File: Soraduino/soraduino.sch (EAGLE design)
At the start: 21 parts, among them IC1 ATMEGA168-AU, IC2 317EMP, IC3 317EMP

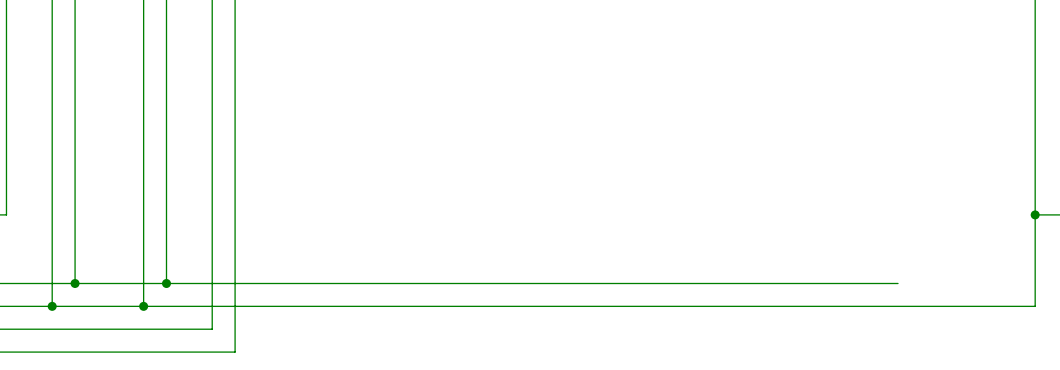
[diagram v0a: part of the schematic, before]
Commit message: 仮配線完了
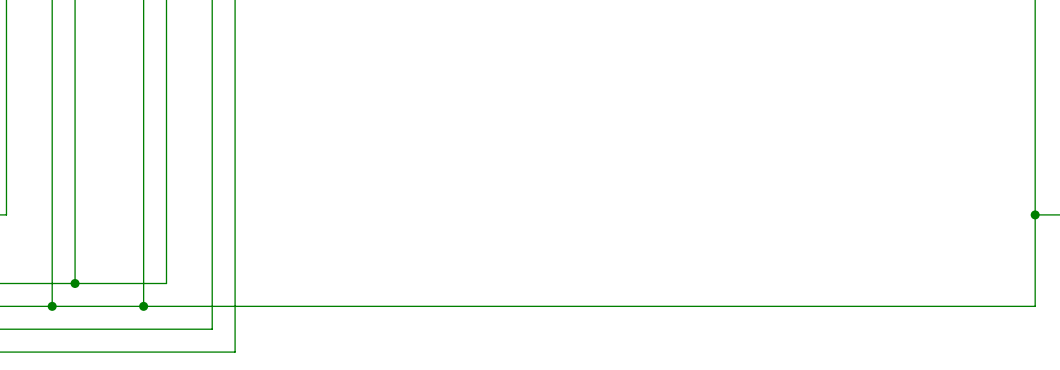
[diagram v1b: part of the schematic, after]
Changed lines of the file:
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@@
 <wire x1="172.72" y1="0" x2="162.56" y2="0" width="0.1524" layer="91"/>
 <junction x="162.56" y="0"/>
-<junction x="172.72" y="0"/>
 <pinref part="IC4" gate="G$1" pin="DCPROG"/>
 <wire x1="137.16" y1="86.36" x2="162.56" y2="86.36" width="0.1524" layer="91"/>
 <junction x="162.56" y="86.36"/>
-<wire x1="172.72" y1="0" x2="254" y2="0" width="0.1524" layer="91"/>
 <pinref part="JAIRO-ANA" gate="G$1" pin="2"/>
 </segment>
@@
 </sheet>
 </sheets>
+<errors>
+</errors>
 </schematic>
 </drawing>

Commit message: back GPS 1
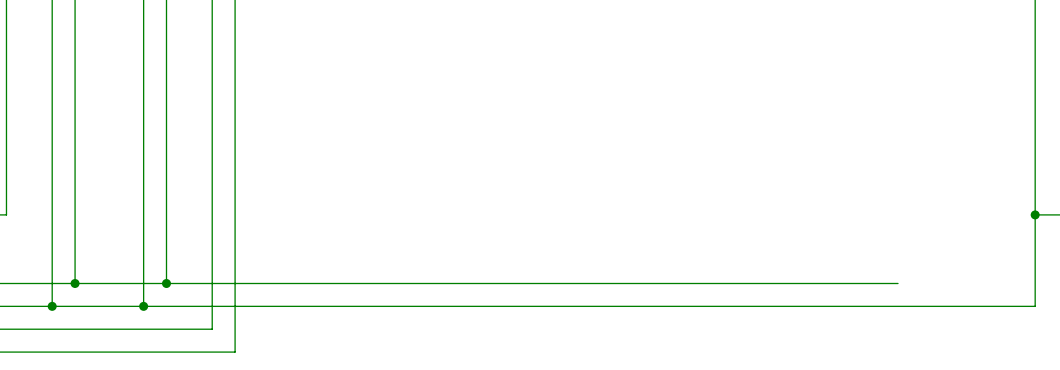
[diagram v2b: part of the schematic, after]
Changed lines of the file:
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@@
 <wire x1="172.72" y1="0" x2="162.56" y2="0" width="0.1524" layer="91"/>
 <junction x="162.56" y="0"/>
+<junction x="172.72" y="0"/>
 <pinref part="IC4" gate="G$1" pin="DCPROG"/>
 <wire x1="137.16" y1="86.36" x2="162.56" y2="86.36" width="0.1524" layer="91"/>
 <junction x="162.56" y="86.36"/>
+<wire x1="172.72" y1="0" x2="254" y2="0" width="0.1524" layer="91"/>
 <pinref part="JAIRO-ANA" gate="G$1" pin="2"/>
 </segment>
@@
 </sheet>
 </sheets>
-<errors>
-</errors>
 </schematic>
 </drawing>
